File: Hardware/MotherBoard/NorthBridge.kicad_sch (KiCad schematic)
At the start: 4 parts, among them U6 74HC148, U7 74HC574, U8 ATF16V8B

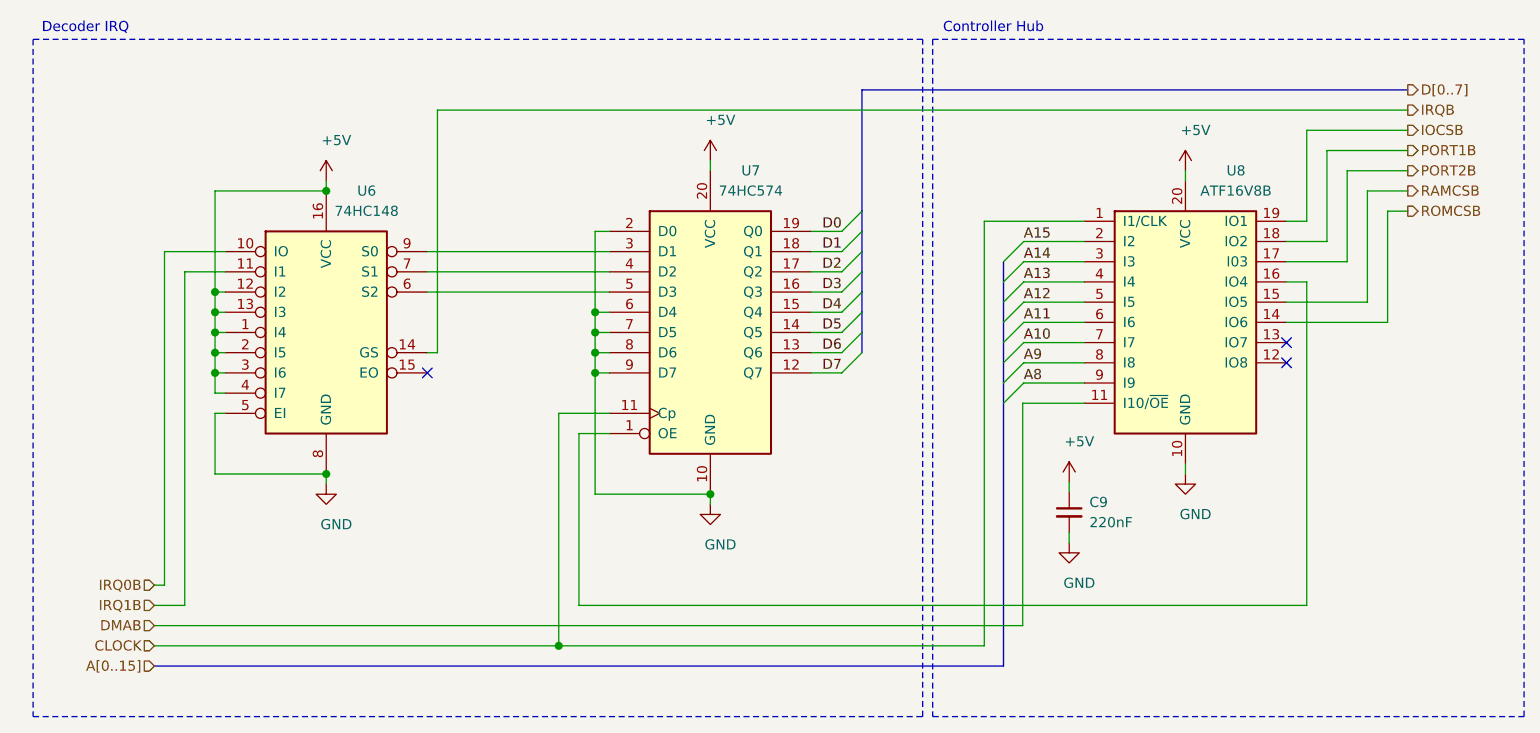
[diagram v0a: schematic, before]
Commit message: Fix
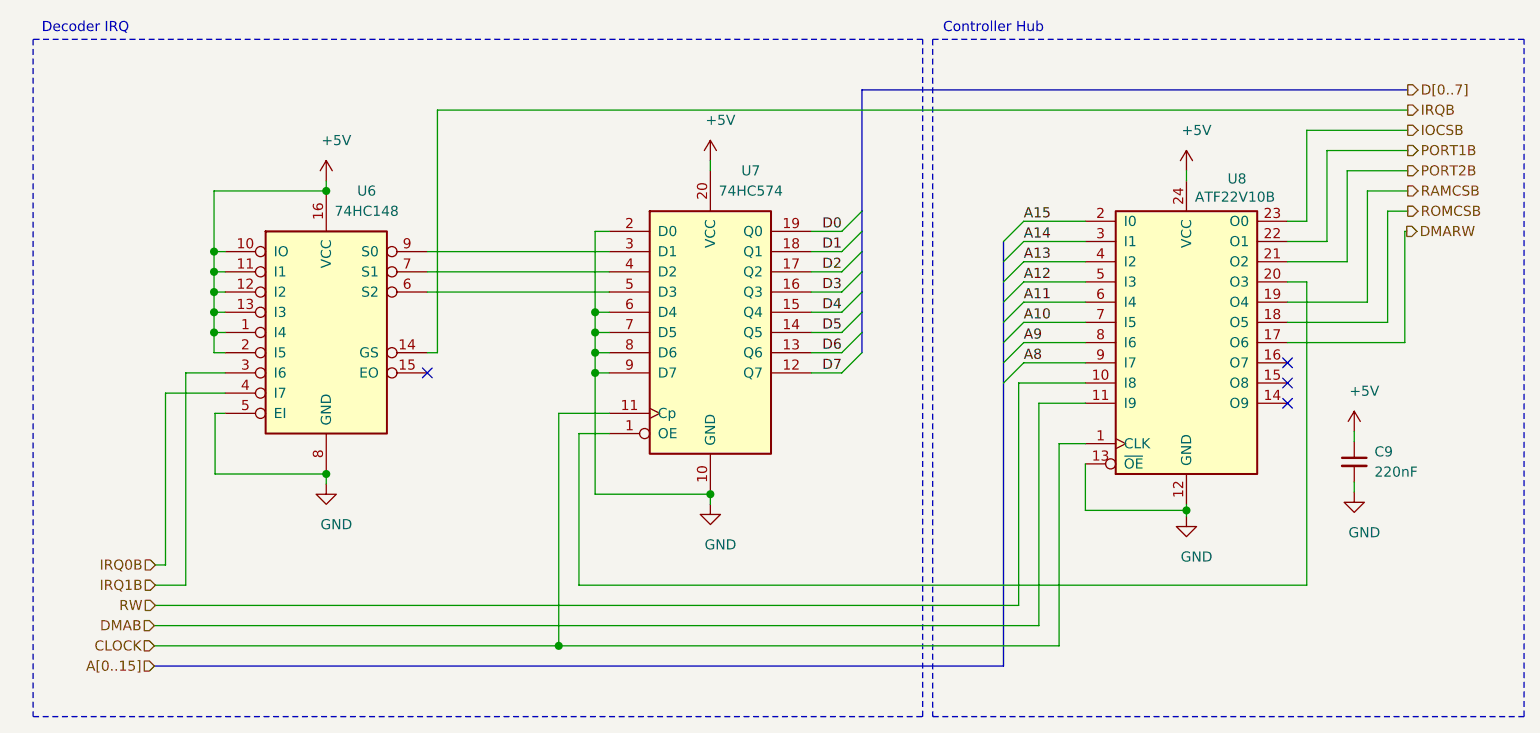
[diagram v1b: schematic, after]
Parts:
- removed U8: ATF16V8B, Package_DIP:DIP-20_W7.62mm, symbol Logic_Programmable:GAL16V8
- added U8: ATF22V10B, Package_DIP:DIP-24_W7.62mm, symbol Logic_Programmable:PAL20RS10
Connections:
- net +5V: now also U6.10 (IO), U6.11 (I1), U8.24 (VCC); no longer U6.3 (I6), U6.4 (I7)
- net A10: now also U8.7 (I5)
- net A11: now also U8.6 (I4)
- net A12: now also U8.5 (I3)
- net A13: now also U8.4 (I2)
- net A14: now also U8.3 (I1)
- net A15: now also U8.2 (I0)
- net A8: now also U8.9 (I7)
- net A9: now also U8.8 (I6)
- net CLOCK: now also U8.1 (CLK)
- net DMAB: now also U8.11 (I9)
- net GND: now also U8.12 (GND), U8.13 (~OE~)
- net IOCSB: now also U8.23 (O0)
- net IRQ0B: now also U6.4 (I7); no longer U6.10 (IO)
- net IRQ1B: now also U6.3 (I6); no longer U6.11 (I1)
- net PORT1B: now also U8.22 (O1)
- net PORT2B: now also U8.21 (O2)
- net RAMCSB: now also U8.19 (O4)
- net ROMCSB: now also U8.18 (O5)
- net at U7.1 (OE): now also U8.20 (O3)
- new net DMARW: U8.17 (O6)
- new net RW: U8.10 (I8)
- no-connect marks 3 -> 4
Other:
- title: Retro 6502 Mother Board -> Miniish
- moved on the sheet: C9
